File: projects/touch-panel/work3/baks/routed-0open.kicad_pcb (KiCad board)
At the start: 2 copper layers, 71 x 150 mm, 269 parts, among them J1 FPC-40P-0.5mm, Q1 AO3400, Q10 AO3400, Q100 AO3400, Q101 AO3400, Q102 AO3400, Q103 AO3400, Q104 AO3400, Q105 AO3400, Q106 AO3400, Q107 AO3400, Q108 AO3400, Q109 AO3400, Q11 AO3400, Q110 AO3400, Q111 AO3400, Q112 AO3400, Q113 AO3400, Q114 AO3400, Q115 AO3400, Q116 AO3400, Q117 AO3400, Q118 AO3400, Q119 AO3400, Q12 AO3400, Q120 AO3400, Q121 AO3400, Q122 AO3400, Q123 AO3400, Q124 AO3400, Q125 AO3400, Q126 AO3400, Q127 AO3400, Q128 AO3400, Q129 AO3400, Q13 AO3400, Q130 AO3400, Q131 AO3400, Q132 AO3400, Q133 AO3400, Q134 AO3400, Q135 AO3400, Q136 AO3400, Q137 AO3400, Q138 AO3400, Q139 AO3400, Q14 AO3400, Q140 AO3400, Q141 AO3400, Q142 AO3400, Q143 AO3400, Q144 AO3400, Q145 AO3400, Q146 AO3400, Q147 AO3400, Q148 AO3400, Q149 AO3400, Q15 AO3400, Q150 AO3400, Q151 AO3400, Q152 AO3400, Q153 AO3400, Q154 AO3400, Q155 AO3400, Q156 AO3400, Q157 AO3400, Q158 AO3400, Q159 AO3400, Q16 AO3400, Q160 AO3400, Q161 AO3400, Q162 AO3400, Q163 AO3400, Q164 AO3400, Q165 AO3400, Q166 AO3400, Q167 AO3400, Q168 AO3400, Q169 AO3400, Q17 AO3400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

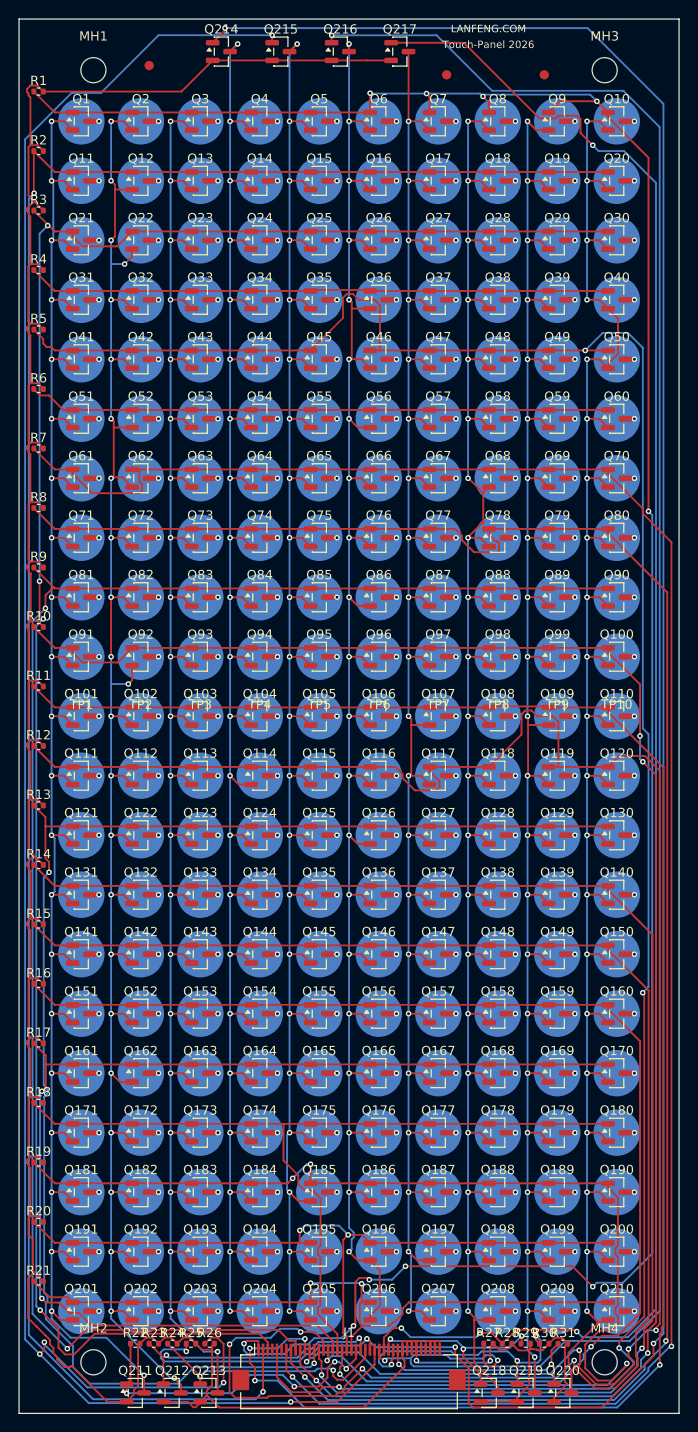
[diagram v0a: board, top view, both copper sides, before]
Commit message: touch-panel完成work3
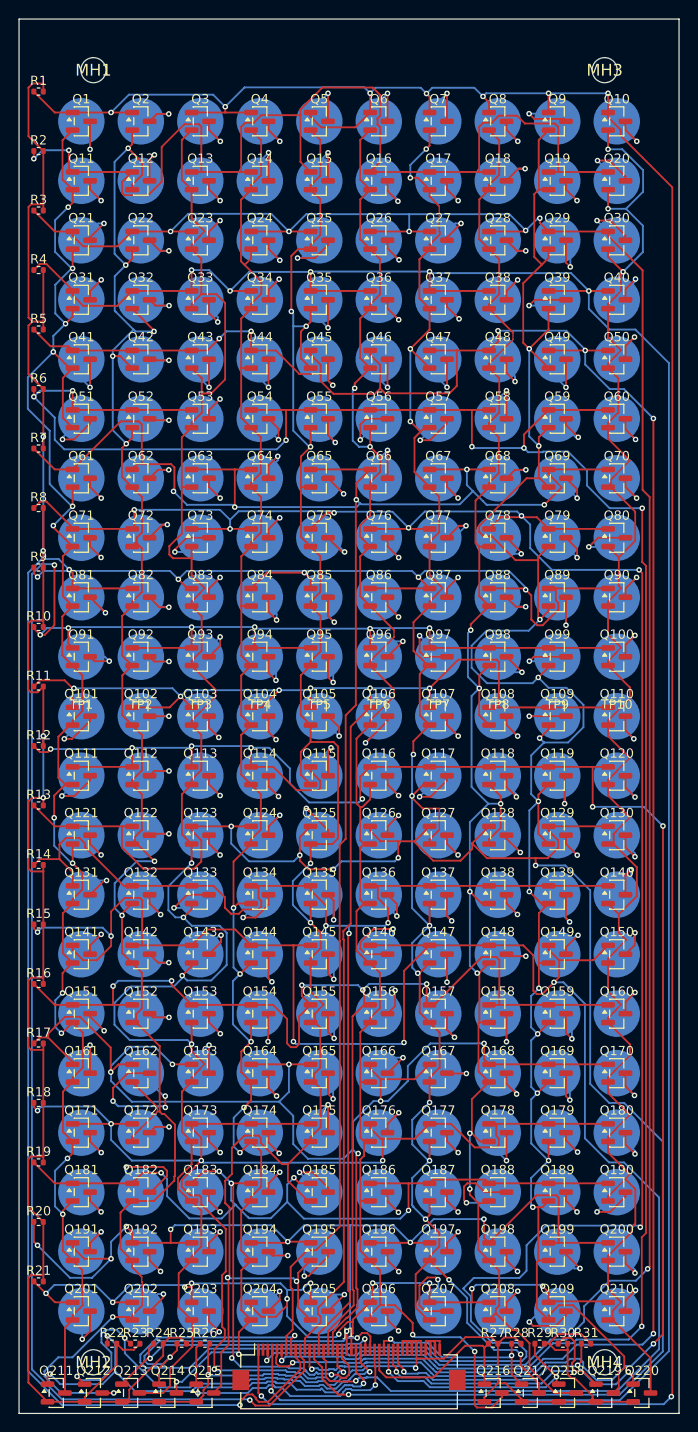
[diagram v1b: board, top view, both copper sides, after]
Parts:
- removed MK1, MK2, MK3: Fiducial_1mm_Mask2mm, 
- moved Q216 145.2 mm to (151.0, 247.8)
- moved Q217 145.0 mm to (155.0, 247.8)
- moved Q215 144.5 mm to (120.0, 247.8)
- moved Q214 144.4 mm to (116.0, 247.8)
- moved Q211 8.51 mm to (104.0, 247.8)
- moved Q220 8.51 mm to (167.0, 247.8)
- moved Q212 8.46 mm to (108.0, 247.8)
- moved Q219 8.46 mm to (163.0, 247.8)
- moved Q213 8.42 mm to (112.0, 247.8)
- moved Q218 8.42 mm to (159.0, 247.8)
- moved R22 2.50 mm to (110.0, 242.5)
- moved R31 2.50 mm to (161.0, 242.5)
- moved R23 2.00 mm to (112.5, 242.5)
- moved R30 2.00 mm to (158.5, 242.5)
- moved R24 1.50 mm to (115.0, 242.5)
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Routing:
- net CSEL3: track 255.8 -> 35.8 mm, vias 5 -> 2
- net CSEL4: track 234.7 -> 29.9 mm, vias 5 -> 2
- net ROW3: track 62.8 -> 262.5 mm, vias 0 -> 6
- net CSEL5: track 216.1 -> 19.9 mm, vias 3 -> 0
- net ROW5: track 62.7 -> 249.1 mm, vias 0 -> 8
- net CSEL6: track 191.3 -> 20.5 mm, vias 4 -> 2
- net ROW1: track 223.2 -> 118.1 mm
- net ROW7: track 204.7 -> 275.9 mm, vias 2 -> 8
- net ROW8: track 173.9 -> 230.6 mm, vias 2 -> 7
- net ROW17: track 90.4 -> 144.2 mm, vias 0 -> 6
- net ROW12: track 152.6 -> 204.5 mm, vias 2 -> 6
- net ROW19: track 78.9 -> 119.4 mm, vias 2 -> 8
- net ROW2: track 211.9 -> 251.9 mm, vias 4 -> 7
- net ROW9: track 185.5 -> 218.4 mm, vias 4 -> 8
- net ROW10: track 194.0 -> 162.2 mm, vias 4 -> 6
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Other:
- board text removed: "LANFENG.COM"
- board text removed: "Touch-Panel 2026"
